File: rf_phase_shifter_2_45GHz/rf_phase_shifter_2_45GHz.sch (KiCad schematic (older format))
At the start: 12 parts, among them J1 Conn_Coaxial, J2 Conn_Coaxial, J3 Conn_Coaxial

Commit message: update
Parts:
- removed FL1: C2327J5003AHF, C2327J5003AHF, symbol RF:C2327J5003AHF
- added FL1: C2327J5003AHF, analog_rf_phase_shifter_module:C2327J5003AHF, symbol analog_rf_phase_shifter_module:C2327J5003AHF
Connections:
- net GND: now also FL1.2 (GND_1), FL1.5 (GND_2)
- net at D1.1 (K), D3.1 (K), L1.2: now also FL1.6 (COUPLED)
- net at D2.1 (K), D4.1 (K), L2.2: now also FL1.4 (DIRECT)
- net at C1.1: now also FL1.1 (INPUT)
- net at C2.2: now also FL1.3 (ISOLATED)
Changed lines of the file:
@@
 EELAYER 30 0
 EELAYER END
-$Descr A4 11693 8268
+$Descr User 8268 5827
 encoding utf-8
 Sheet 1 1
-Title ""
-Date ""
-Rev ""
-Comp ""
+Title "Analog RF phase shifter 2,4-2,5GHz"
+Date "2021-05-03"
+Rev "1.0.0"
+Comp "Marcin Wachowiak, Poland"
 Comment1 ""
 Comment2 ""
@@
 	4450 1950 4450 1900
 Connection ~ 3900 1900
-$Comp
-L RF:C2327J5003AHF FL1
-U 1 1 60586F9C
-P 2200 1700
-F 0 "FL1" H 2950 1965 50  0000 C CNN
-F 1 "C2327J5003AHF" H 2950 1874 50  0000 C CNN
-F 2 "C2327J5003AHF" H 3550 1800 50  0001 L CNN
-F 3 "https://componentsearchengine.com/Datasheets/1/C2327J5003AHF.pdf" H 3550 1700 50  0001 L CNN
-F 4 "Signal Conditioning 2.3-2.7GHz IL=.4dB 3dB 90 Deg." H 3550 1600 50  0001 L CNN "Description"
-F 5 "0.73" H 3550 1500 50  0001 L CNN "Height"
-F 6 "ANAREN" H 3550 1400 50  0001 L CNN "Manufacturer_Name"
-F 7 "C2327J5003AHF" H 3550 1300 50  0001 L CNN "Manufacturer_Part_Number"
-F 8 "620-C2327J5003AHF" H 3550 1200 50  0001 L CNN "Mouser Part Number"
-F 9 "https://www.mouser.com/Search/Refine.aspx?Keyword=620-C2327J5003AHF" H 3550 1100 50  0001 L CNN "Mouser Price/Stock"
-	1    2200 1700
-	1    0    0    -1
-$EndComp
 Wire Wire Line
 	5000 2250 5000 2300
@@
 Wire Notes Line
 	4000 1950 4300 1950
+$Comp
+L analog_rf_phase_shifter_module:C2327J5003AHF FL1
+U 1 1 6090630C
+P 2200 1700
+F 0 "FL1" H 2950 1965 50  0000 C CNN
+F 1 "C2327J5003AHF" H 2950 1874 50  0000 C CNN
+F 2 "analog_rf_phase_shifter_module:C2327J5003AHF" H 3550 1800 50  0001 L CNN
+F 3 "https://componentsearchengine.com/Datasheets/1/C2327J5003AHF.pdf" H 3550 1700 50  0001 L CNN
+F 4 "Signal Conditioning 2.3-2.7GHz IL=.4dB 3dB 90 Deg." H 3550 1600 50  0001 L CNN "Description"
+F 5 "0.73" H 3550 1500 50  0001 L CNN "Height"
+F 6 "ANAREN" H 3550 1400 50  0001 L CNN "Manufacturer_Name"
+F 7 "C2327J5003AHF" H 3550 1300 50  0001 L CNN "Manufacturer_Part_Number"
+	1    2200 1700
+	1    0    0    -1
+$EndComp
 $EndSCHEMATC

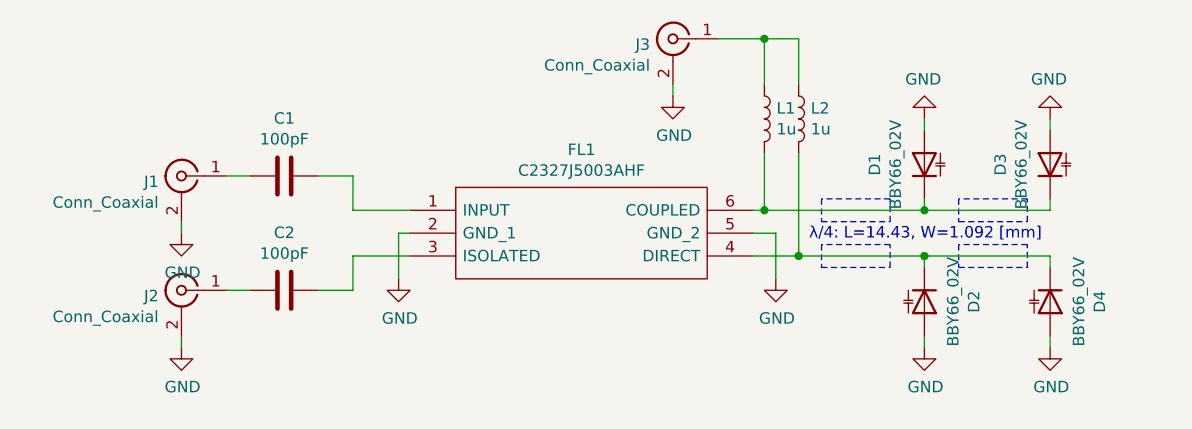
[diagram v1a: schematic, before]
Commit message: updated libs
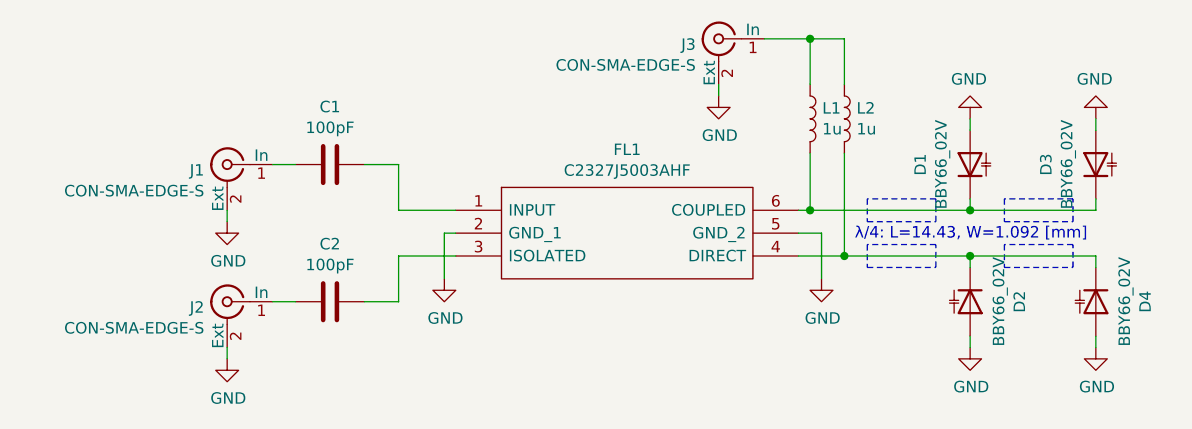
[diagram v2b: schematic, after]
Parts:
- removed J1, J2, J3: Conn_Coaxial, Connector_Coaxial:SMA_Samtec_SMA-J-P-X-ST-EM1_EdgeMount, symbol Connector:Conn_Coaxial
- added J1, J2, J3: CON-SMA-EDGE-S, analog_rf_phase_shifter_module:CON-SMA-EDGE-S, symbol analog_rf_phase_shifter_module:CON-SMA-EDGE-S
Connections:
- net GND: now also J1.2 (Ext), J2.2 (Ext), J3.2 (Ext)
- net at L1.1, L2.1: now also J3.1 (In)
- net at C2.1: now also J2.1 (In)
- net at C1.2: now also J1.1 (In)
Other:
- moved on the sheet: C1, C2, D1, D2, D3, D4, FL1, L1, L2
